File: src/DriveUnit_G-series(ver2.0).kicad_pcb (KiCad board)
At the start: 2 copper layers, 65.7 x 23.3 mm, 52 parts, among them IC1 A3921, Q1 SQJA16EP-T1_GE3, Q2 SQJA16EP-T1_GE3, Q3 SQJA16EP-T1_GE3, Q4 SQJA16EP-T1_GE3, Q5 Q_NPN_BCE, Q6 Q_NPN_BCE, SW3 THAF01-NC-R, U2 TC7S14F

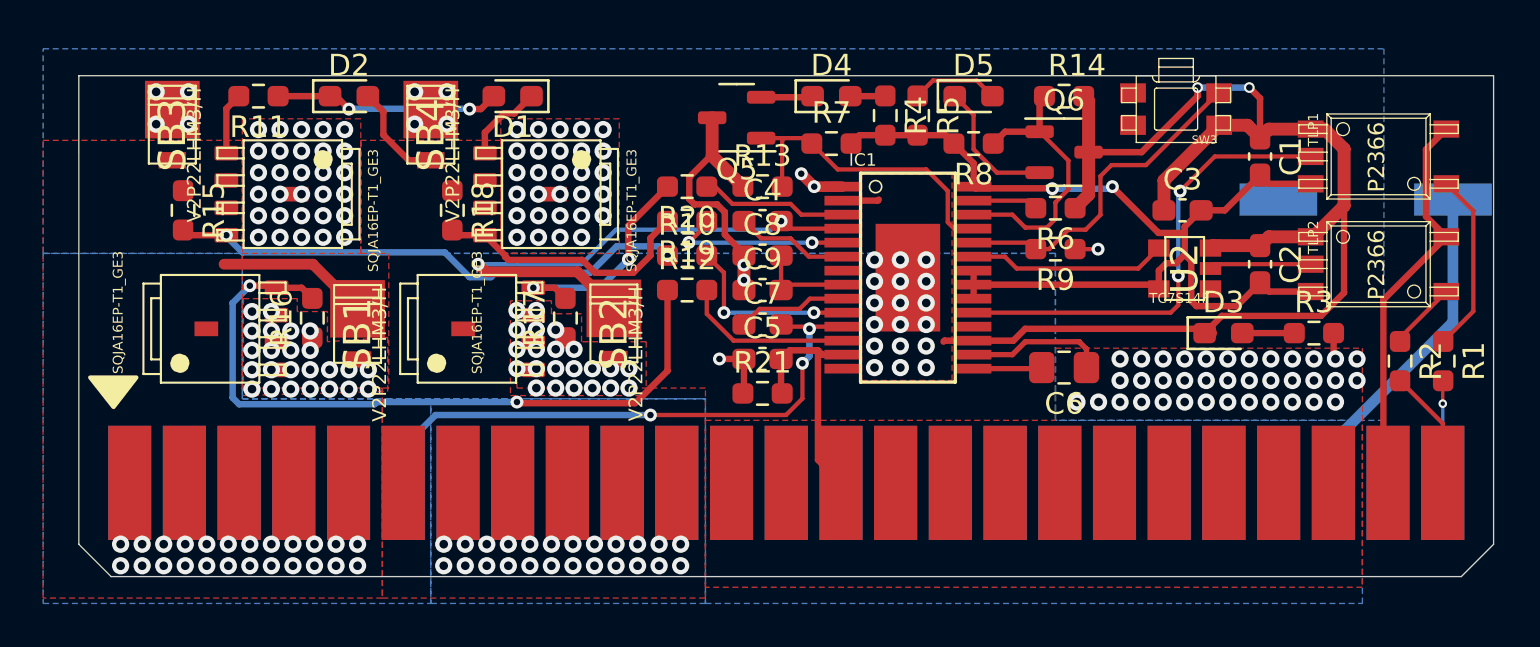
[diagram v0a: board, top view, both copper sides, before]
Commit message: [wip]DRC全通過完了
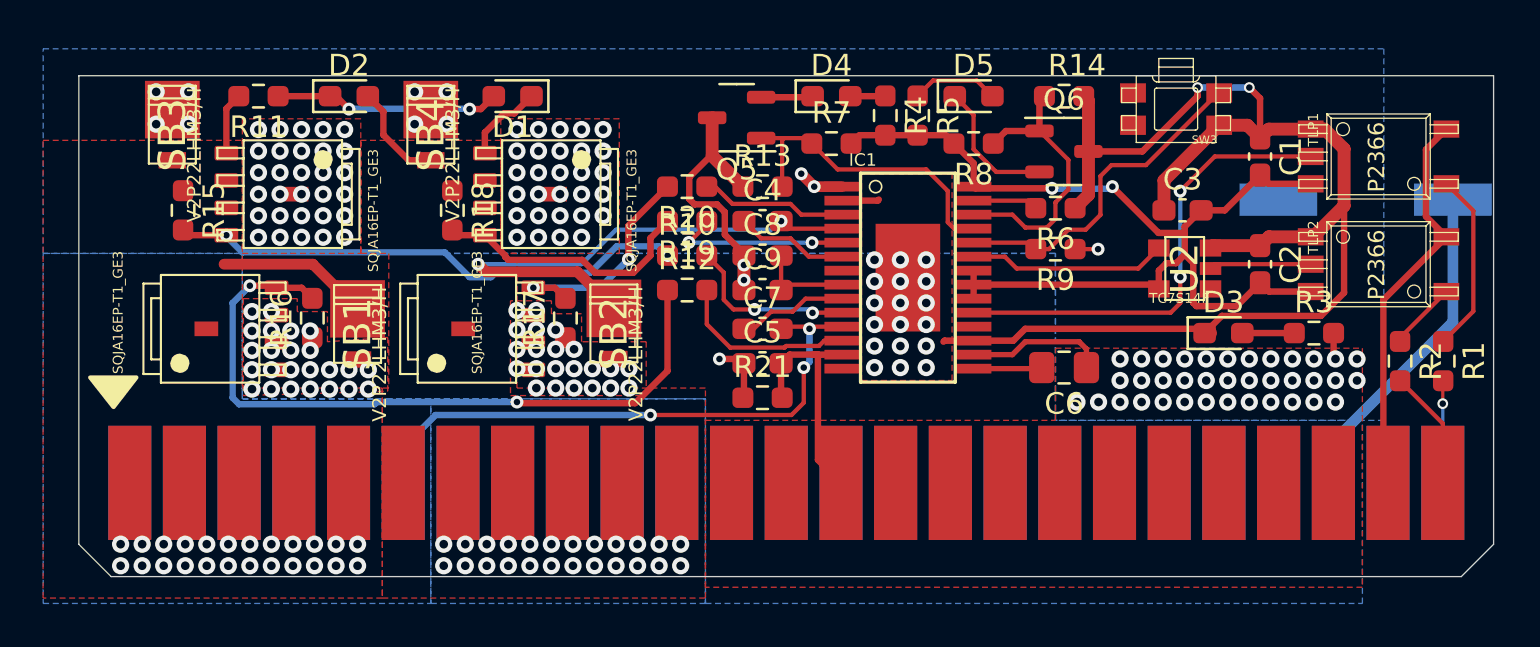
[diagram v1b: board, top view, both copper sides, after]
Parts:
- moved C7 0.20 mm to (147.4, 119.0)
- moved R21 0.20 mm to (147.4, 122.2)
- moved C5 0.20 mm to (147.4, 120.6)
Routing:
- net /GLA: track 7.91 -> 8.46 mm

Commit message: :tada:完成
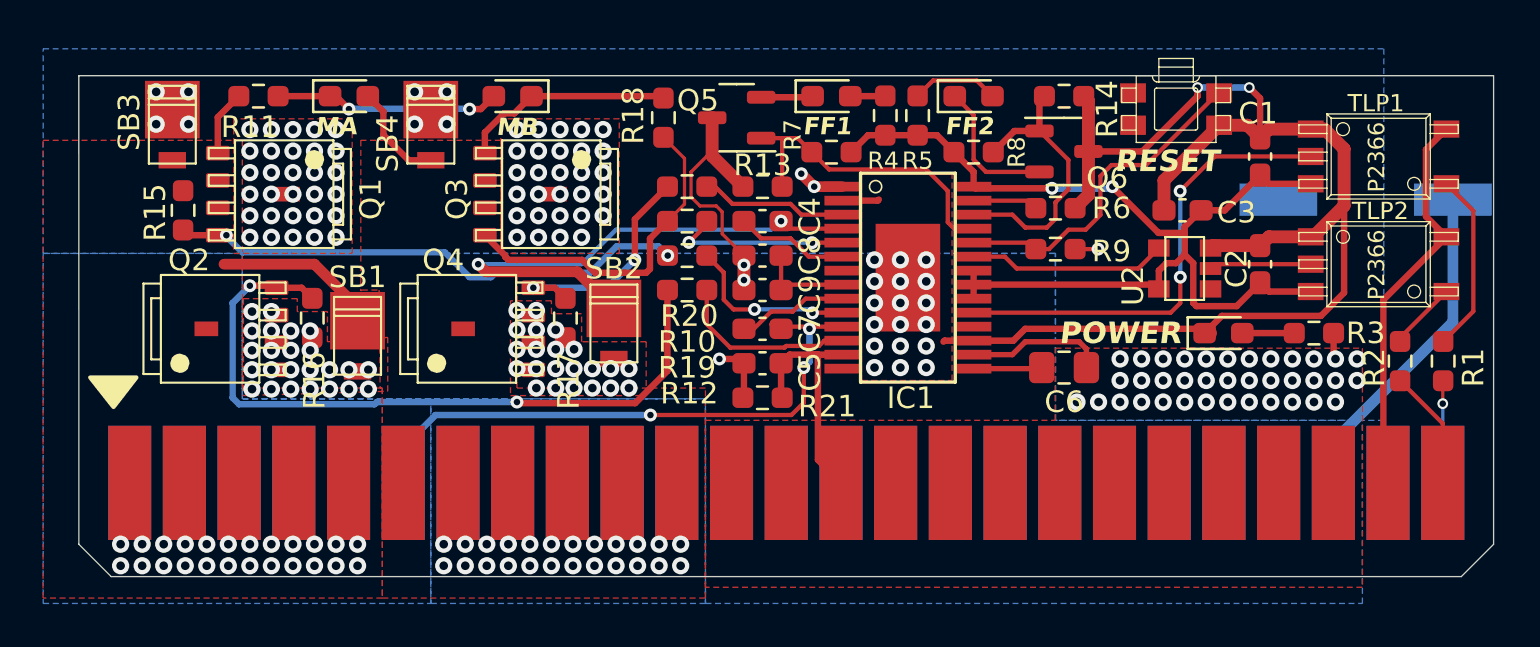
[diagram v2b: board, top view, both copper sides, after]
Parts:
- added G***: LOGO, LOGO, B.Cu at (139.6, 119.4)
- added G***: LOGO, LOGO, B.Cu at (156.4, 114.0)
- moved R18 10.7 mm to (142.8, 109.2)
- moved SB1 0.55 mm to (128.6, 119.8)
- moved Q1 0.40 mm to (124.1, 112.8)
- moved R7 0.40 mm to (150.6, 110.8)
- moved R8 0.40 mm to (157.2, 110.8)
- renumbered D4 to FF1, D5 to FF2, D2 to MA, D1 to MB, D3 to POWER, SW3 to RESET
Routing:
- net /SB: track 33.6 -> 39.8 mm
- net Net-(Q3-PadG): track 12.3 -> 15.7 mm
- net /SA: track 38.0 -> 38.8 mm
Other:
- board text added: "53"
- board text added: "HOW TO USE"
- board text added: "MOEL"
- board text added: "Note:"
- board text added: "ver 1.0"
